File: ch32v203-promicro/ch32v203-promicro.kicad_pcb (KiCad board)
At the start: 2 copper layers, 17.8 x 33 mm, 27 parts, among them J1 USB2.0_C_v3, J2 ProMicro-LeftPin, J3 ProMicro-RightPin, SW1 SW_Push, SW2 SW_Push, U1 CH32V203CxT6, U2 AMS1117-3.3, Y1 32.768k, Y2 8M

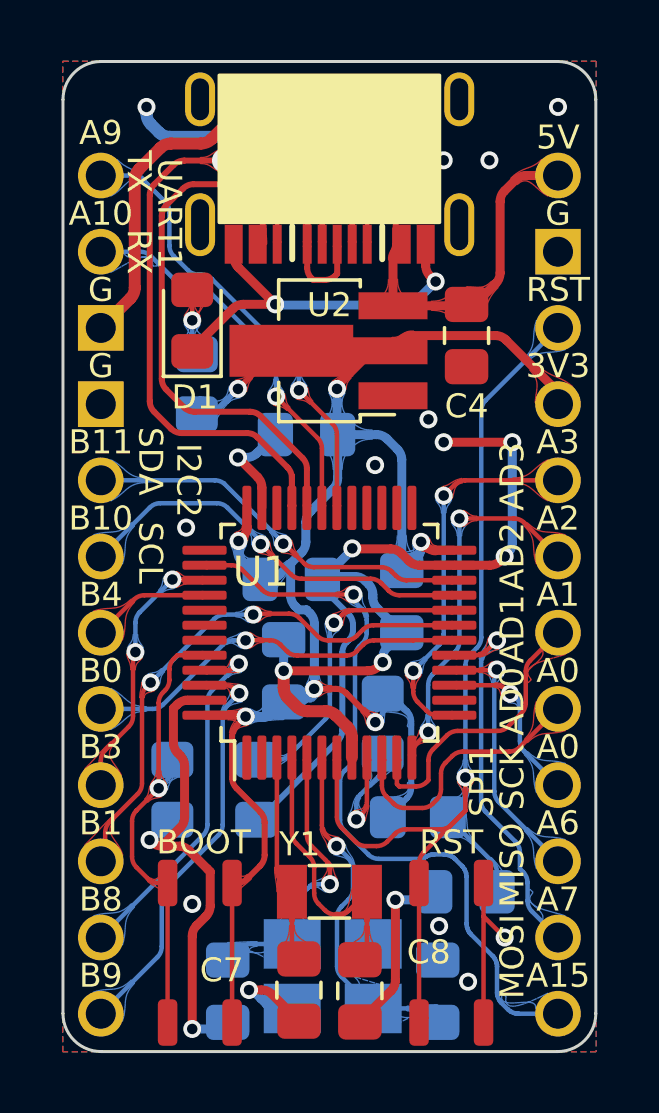
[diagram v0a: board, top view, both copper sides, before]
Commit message: stm32
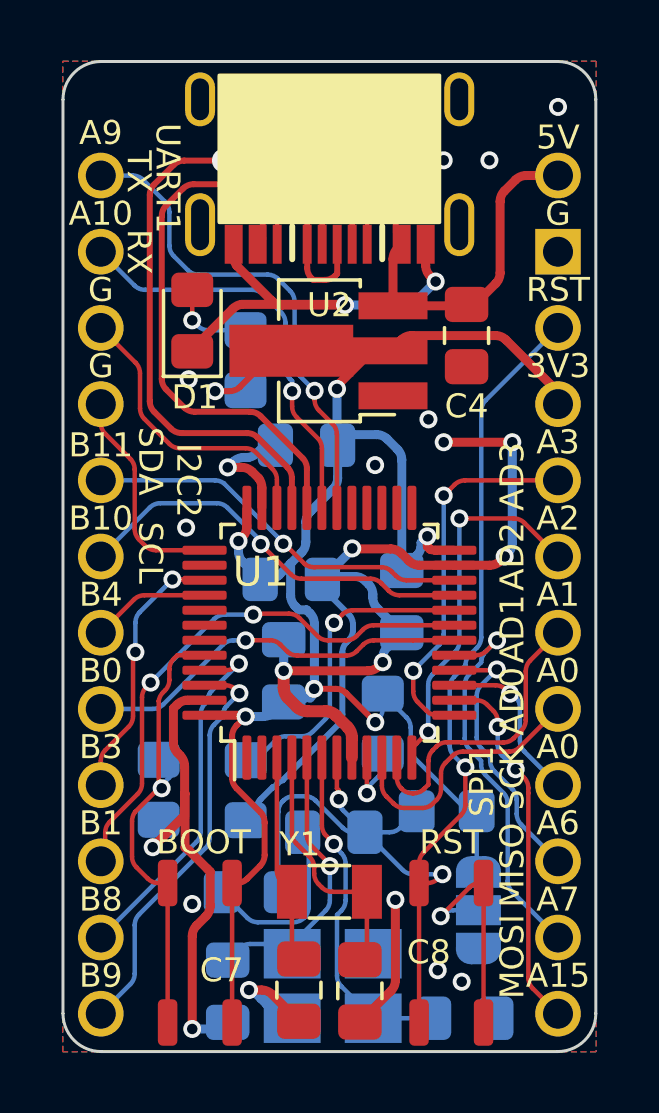
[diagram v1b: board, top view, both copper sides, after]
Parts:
- added JP1: Jumper_3_Open, Jumper:SolderJumper-3_P1.3mm_Open_RoundedPad1.0x1.5mm, B.Cu at (113.9, 128.3)
- added R8: 10k, $74th:Register_0805_2012, B.Cu at (106.2, 127.6)
- J2: value ProMicro-LeftPin -> ProMicro-LeftPin-NoGND; footprint $74th:ProMicro_LIKE_LEFT -> $74th:ProMicro_LIKE_LEFT_NO_GND
- moved C6 4.83 mm to (109.0, 125.7)
- moved R1 1.81 mm to (106.2, 109.9)
- moved C10 1.27 mm to (113.4, 131.9), turned to 0 degrees
- moved R2 0.86 mm to (112.7, 124.9), turned to 180 degrees
- moved R6 0.46 mm to (103.1, 124.4)
- moved C5 0.35 mm to (108.1, 112.8)
- moved R7 0.35 mm to (106.0, 124.4)
- moved Y2 0.32 mm to (109.0, 130.8)
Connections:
- J2 pad 3: GND -> SWDIO
- J2 pad 4: GND -> SWCLK
- SW1 pad 1: GND -> Net-(JP1-C)
- U1 pad 14: unconnected-(U1-Pad14) -> 10/A10
- U1 pad 34: unconnected-(U1-Pad34) -> SWDIO
- U1 pad 37: unconnected-(U1-Pad37) -> SWCLK
- U1 pad 38: 10/A10 -> unconnected-(U1-PA15-Pad38)
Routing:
- net 10/A10: track 25.2 -> 12.3 mm, vias 1 -> 2
- net GND: track 98.7 -> 86.5 mm, vias 25 -> 23
- net SWDIO: track 0.00 -> 9.83 mm
- net Net-(JP1-C): track 0.00 -> 7.83 mm, vias 0 -> 1
- net SWCLK: track 0.00 -> 7.28 mm
- net RST: track 36.6 -> 40.3 mm, vias 1 -> 3
- net +3V3: track 64.4 -> 67.1 mm
- net Net-(U1-VDDA): track 4.69 -> 2.70 mm
- net 1/UART_TX: track 15.2 -> 16.5 mm
- net DP: track 25.5 -> 24.4 mm
- net 0/UART_RX: track 12.8 -> 13.8 mm
- net Net-(D1-A): track 2.19 -> 2.91 mm
- net 19/A1: track 9.64 -> 10.2 mm
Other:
- board text added: "B"
- board text added: "SELECT BOOT0 R2:3V3 R8:GND"
- board text added: "STM32Micro"
- board text added: "V"
- board text removed: "C32V203Micro"
